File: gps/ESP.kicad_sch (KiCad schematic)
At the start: 27 parts, among them J12 ENC+RGB, J13 ENC+RGB, J7 USB_B_Micro, J9 USB_pads, SW1 RotaryEncoder_Switch, U11 SN74LV1T34DBVRG4, U3 DFR0654, U9 TCA39306DDFR

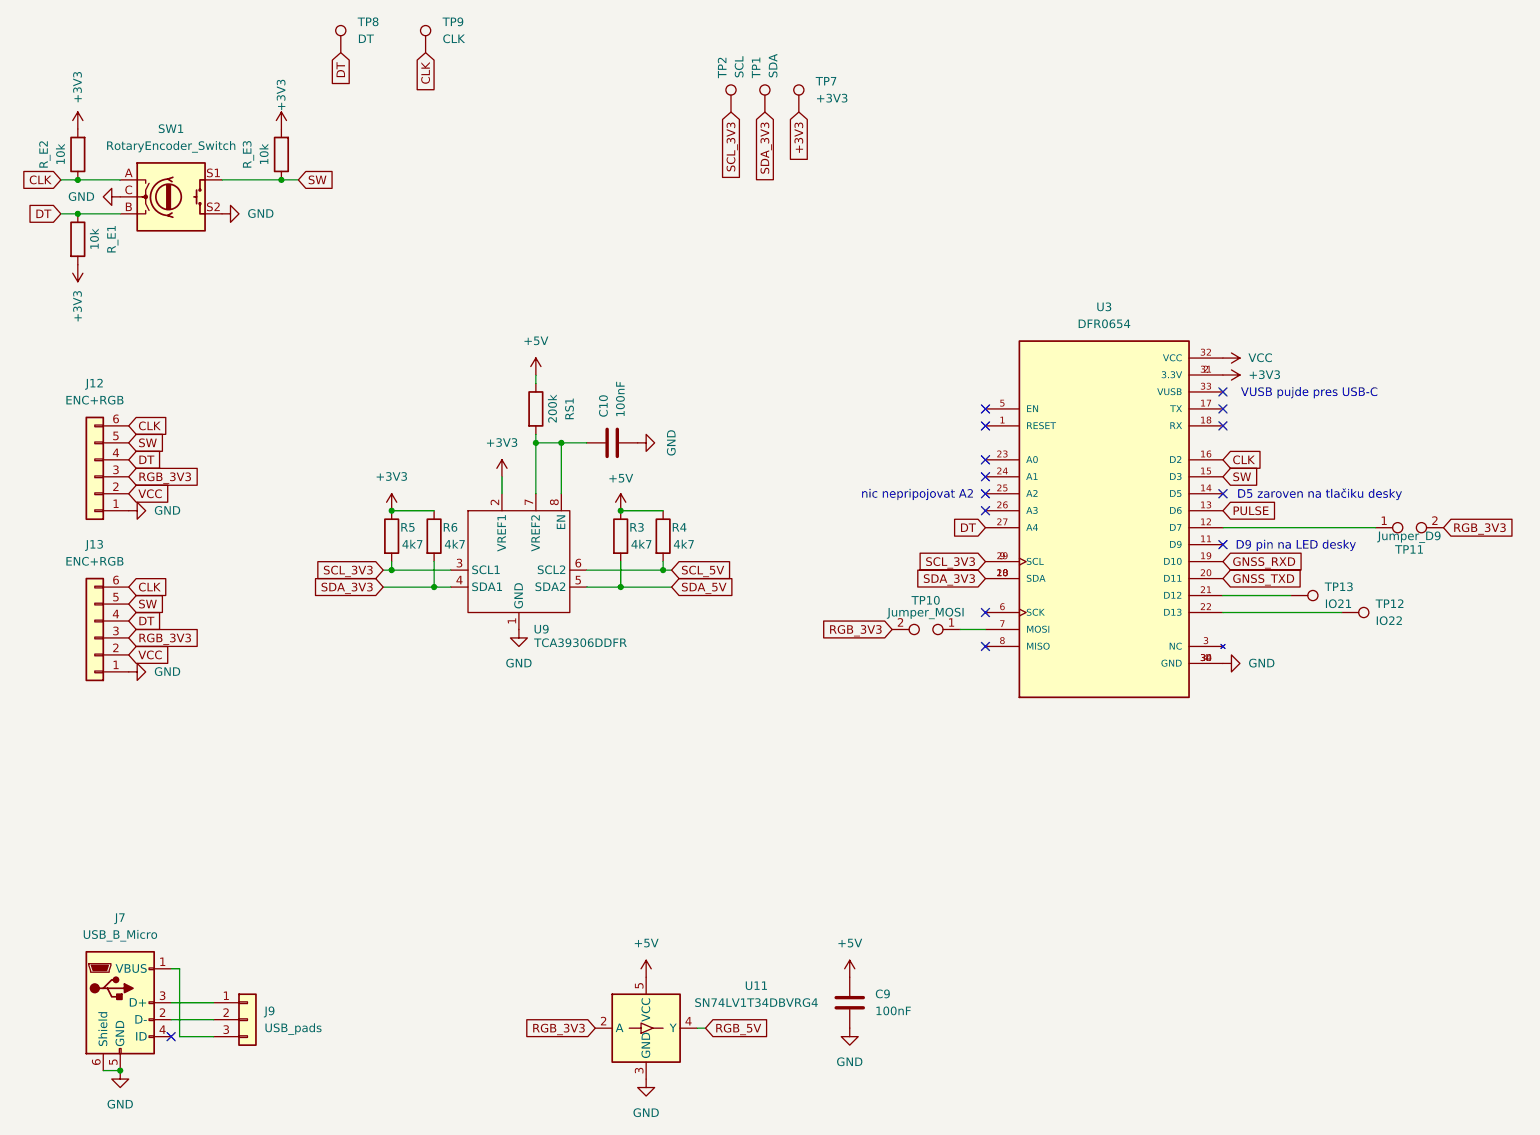
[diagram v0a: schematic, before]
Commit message: cleaned schematic
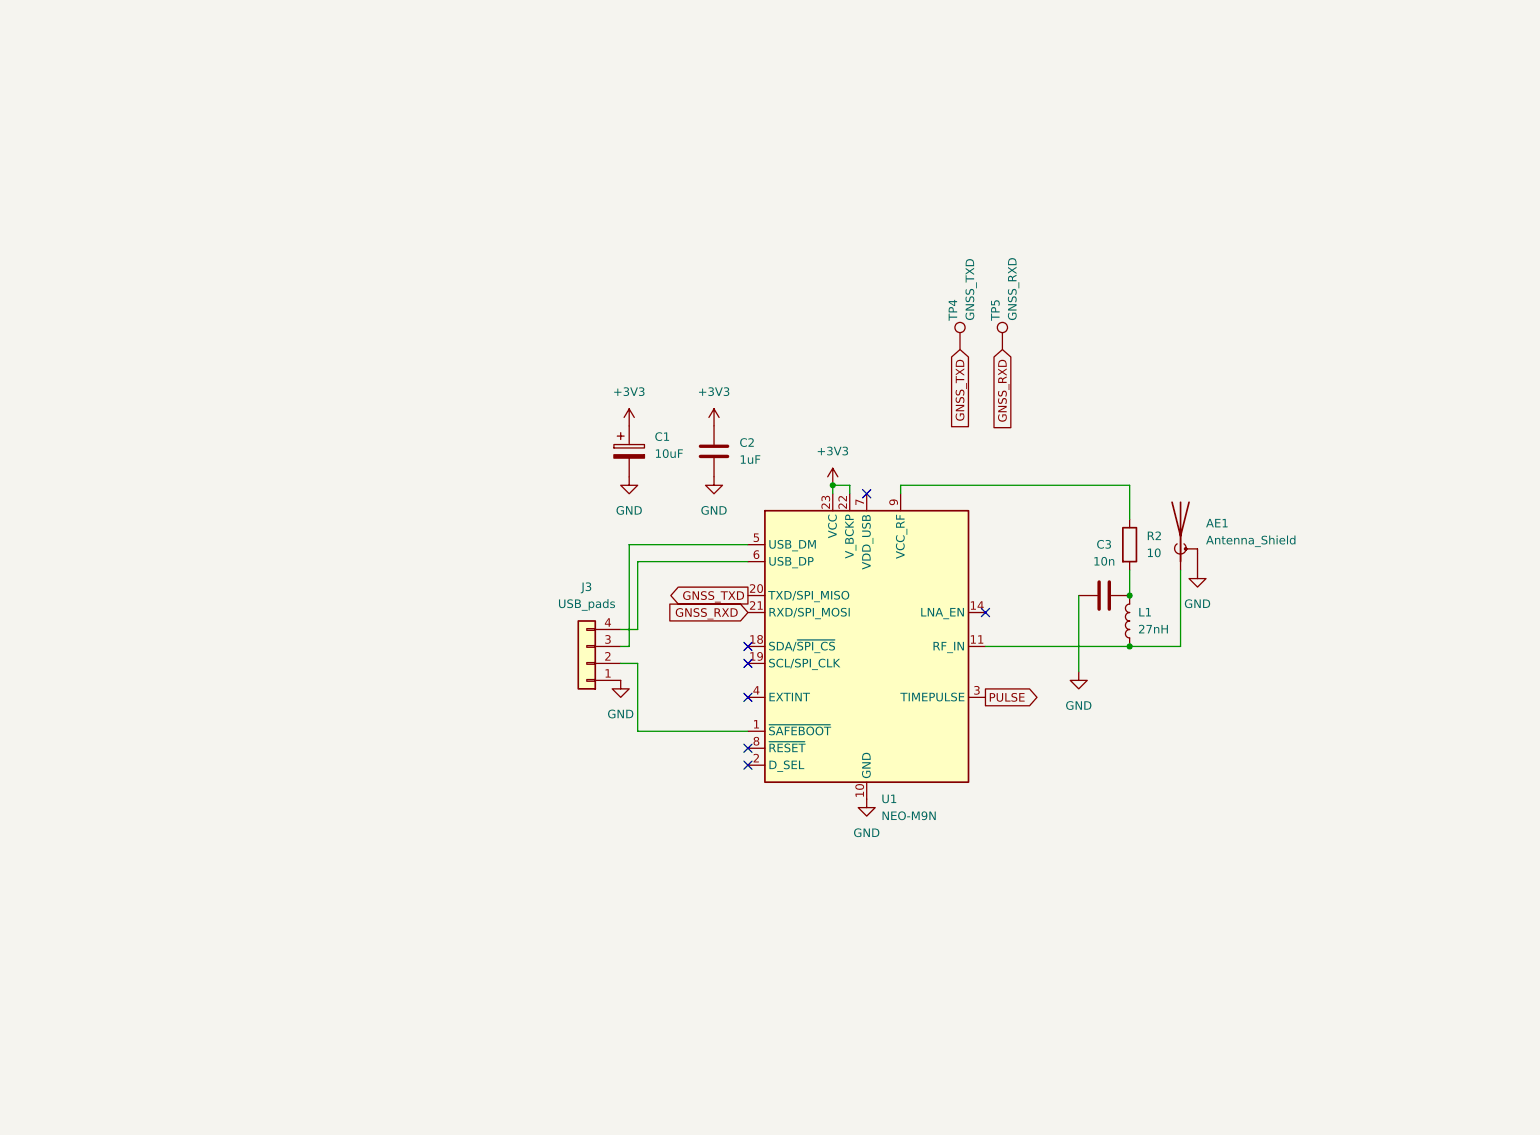
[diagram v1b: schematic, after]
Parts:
- removed C10, C9: 100nF, Capacitor_SMD:C_0805_2012Metric_Pad1.18x1.45mm_HandSolder, symbol Device:C
- removed J12: ENC+RGB, Connector_PinSocket_2.54mm:PinSocket_1x06_P2.54mm_Vertical, symbol Connector_Generic:Conn_01x06
- removed J13: ENC+RGB, Connector_PinHeader_2.54mm:PinHeader_1x06_P2.54mm_Vertical, symbol Connector_Generic:Conn_01x06
- removed J7: USB_B_Micro, KiCad:USB3145301A, symbol Connector:USB_B_Micro
- removed J9: USB_pads, Connector_PinSocket_2.54mm:PinSocket_1x03_P2.54mm_Vertical, symbol Connector_Generic:Conn_01x03
- removed R3, R4, R5, R6: 4k7, Resistor_SMD:R_0805_2012Metric_Pad1.20x1.40mm_HandSolder, symbol Device:R
- removed RS1: 200k, Resistor_SMD:R_0805_2012Metric_Pad1.20x1.40mm_HandSolder, symbol Device:R
- removed R_E1, R_E2, R_E3: 10k, Resistor_SMD:R_0805_2012Metric_Pad1.20x1.40mm_HandSolder, symbol Device:R
- removed SW1: RotaryEncoder_Switch, Rotary_Encoder:RotaryEncoder_20mm_WO_mount_holes, symbol Device:RotaryEncoder_Switch
- removed TP1: SDA, TestPoint:TestPoint_Loop_D1.80mm_Drill1.0mm_Beaded, symbol Connector:TestPoint
- removed TP10: Jumper_MOSI, Resistor_SMD:R_0805_2012Metric_Pad1.20x1.40mm_HandSolder, symbol Connector:TestPoint_2Pole
- removed TP11: Jumper_D9, Resistor_SMD:R_0805_2012Metric_Pad1.20x1.40mm_HandSolder, symbol Connector:TestPoint_2Pole
- removed TP12: IO22, TestPoint:TestPoint_Loop_D1.80mm_Drill1.0mm_Beaded, symbol Connector:TestPoint
- removed TP13: IO21, TestPoint:TestPoint_Loop_D1.80mm_Drill1.0mm_Beaded, symbol Connector:TestPoint
- removed TP2: SCL, TestPoint:TestPoint_Loop_D1.80mm_Drill1.0mm_Beaded, symbol Connector:TestPoint
- removed TP7: +3V3, TestPoint:TestPoint_Loop_D1.80mm_Drill1.0mm_Beaded, symbol Connector:TestPoint
- removed TP8: DT, TestPoint:TestPoint_Loop_D1.80mm_Drill1.0mm_Beaded, symbol Connector:TestPoint
- removed TP9: CLK, TestPoint:TestPoint_Loop_D1.80mm_Drill1.0mm_Beaded, symbol Connector:TestPoint
- removed U11: SN74LV1T34DBVRG4, Package_TO_SOT_SMD:SOT-23-5, symbol Logic_LevelTranslator:SN74LV1T34DBV
- removed U3: DFR0654, DFR0654:DFR0654_2, symbol DFR0654:DFR0654
- removed U9: TCA39306DDFR, Package_TO_SOT_SMD:SOT-23-8, symbol shifter:TCA39306DCURQ1
- added AE1: Antenna_Shield, w_conn_rf:lemo_epb00250ntn, symbol Device:Antenna_Shield
- added C1: 10uF, Capacitor_Tantalum_SMD:CP_EIA-3528-15_AVX-H_Pad1.50x2.35mm_HandSolder, symbol Device:C_Polarized
- added C2: 1uF, Capacitor_SMD:C_0603_1608Metric_Pad1.08x0.95mm_HandSolder, symbol Device:C
- added C3: 10n, Capacitor_SMD:C_0805_2012Metric_Pad1.18x1.45mm_HandSolder, symbol Device:C
- added J3: USB_pads, Connector_PinHeader_2.54mm:PinHeader_1x04_P2.54mm_Vertical, symbol Connector_Generic:Conn_01x04
- added L1: 27nH, Inductor_SMD:L_0402_1005Metric_Pad0.77x0.64mm_HandSolder, symbol Device:L
- added R2: 10, Resistor_SMD:R_1206_3216Metric_Pad1.30x1.75mm_HandSolder, symbol Device:R
- added TP4: GNSS_TXD, TestPoint:TestPoint_Loop_D1.80mm_Drill1.0mm_Beaded, symbol Connector:TestPoint
- added TP5: GNSS_RXD, TestPoint:TestPoint_Loop_D1.80mm_Drill1.0mm_Beaded, symbol Connector:TestPoint
- added U1: NEO-M9N, RF_GPS:ublox_NEO, symbol RF_GPS:NEO-M8N
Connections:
- net +3V3: now also C1.1, C2.1, U1.22 (V_BCKP), U1.23 (VCC)
- net GND: now also AE1.2 (Shield), C1.2, C2.2, C3.1, J3.1 (Pin_1), U1.10 (GND), U1.12 (GND), U1.13 (GND), U1.24 (GND)
- net GNSS_RXD: now also TP5.1, U1.21 (RXD/SPI_MOSI)
- net GNSS_TXD: now also TP4.1, U1.20 (TXD/SPI_MISO)
- net PULSE: now also U1.3 (TIMEPULSE)
- new net: J3.2 (Pin_2), U1.1 (~{SAFEBOOT})
- new net: J3.3 (Pin_3), U1.5 (USB_DM)
- new net: J3.4 (Pin_4), U1.6 (USB_DP)
- new net: AE1.1 (A), L1.1, U1.11 (RF_IN)
- new net: C3.2, L1.2, R2.2
- new net: R2.1, U1.9 (VCC_RF)
- no-connect marks 14 -> 7
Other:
- note removed: "D5 zaroven na tlačiku desky"
- note removed: "D9 pin na LED desky"
- note removed: "VUSB pujde pres USB-C"
- note removed: "nic nepripojovat A2"
